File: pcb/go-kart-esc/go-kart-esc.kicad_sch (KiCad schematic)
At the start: 18 parts, among them J1 VBAT, J103 5V_CONN, J104 CAN_CONN, J105 SWD_CONN, J106 TEMP_CONN_A, J107 ENCODER_CONN_A, J108 ENCODER_CONN_B, J109 TEMP_CONN_B, J111 THROTTLE_CONN, J112 BRAKE_CONN, J3 GND

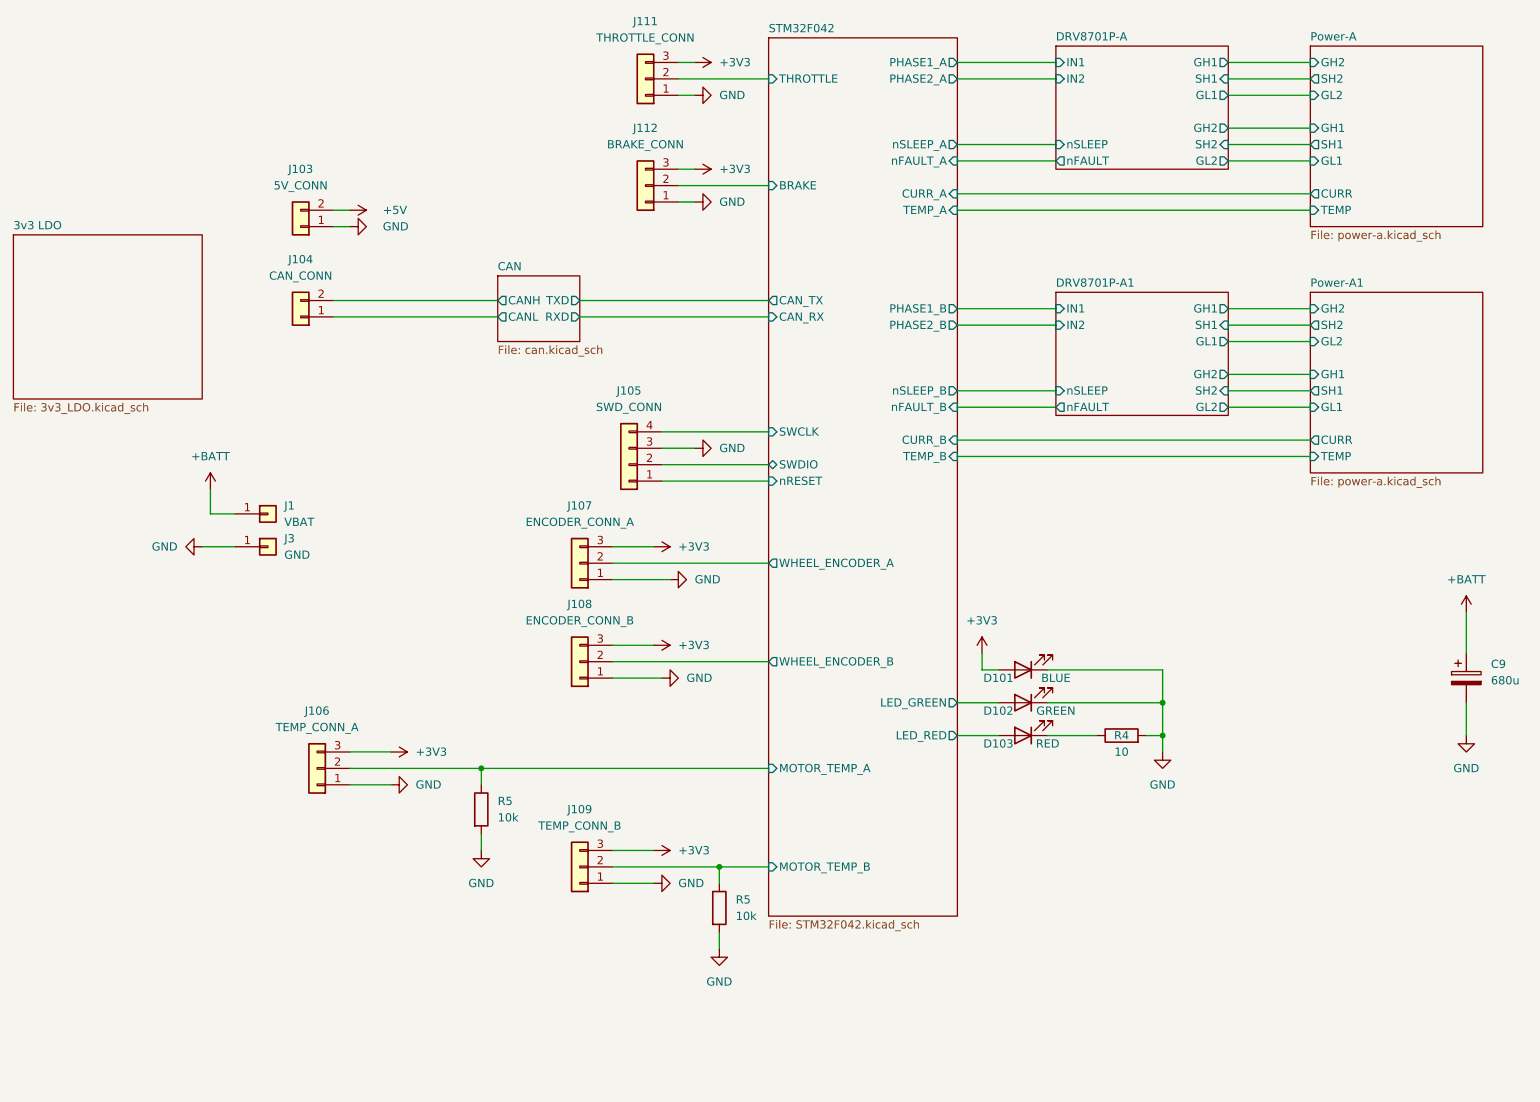
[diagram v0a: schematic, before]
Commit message: Theory can only take you so far.
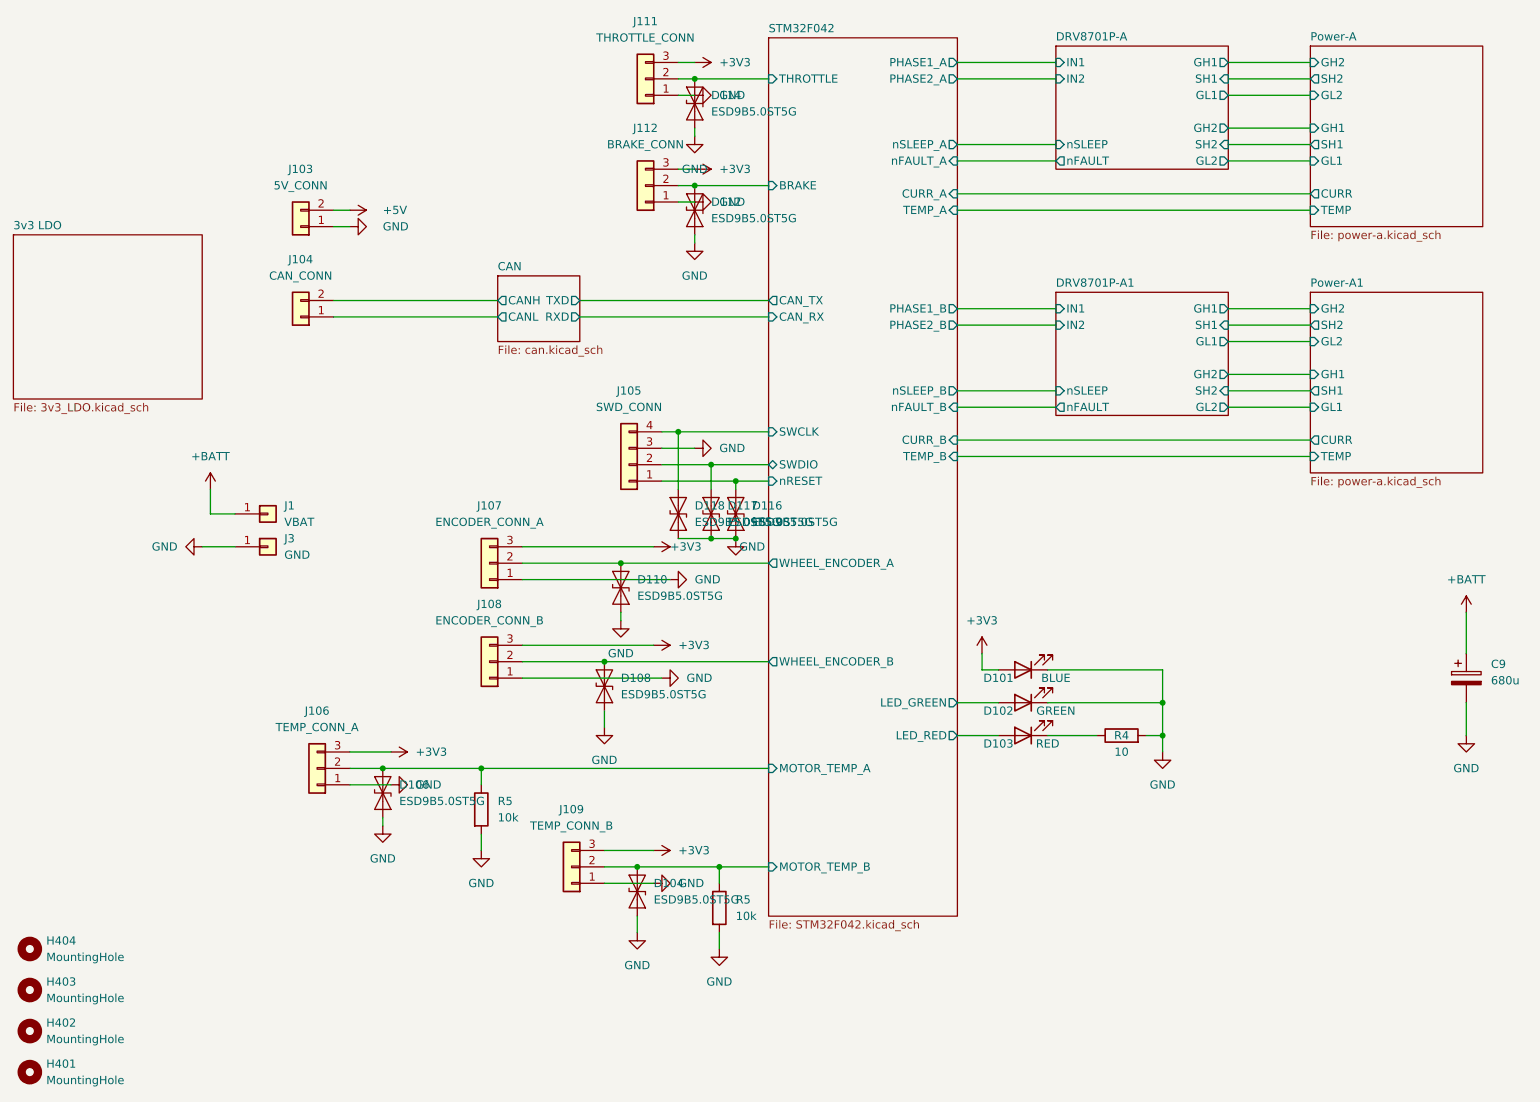
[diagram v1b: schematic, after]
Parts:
- added D104, D106, D108, D110, D112, D114, D116, D117, D118: ESD9B5.0ST5G, Diode_SMD:D_SOD-923, symbol Diode:ESD9B5.0ST5G
- added H401, H402, H403, H404: MountingHole, MountingHole:MountingHole_3.2mm_M3, symbol Mechanical:MountingHole
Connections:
- net GND: now also D104.1 (A1), D106.1 (A1), D108.1 (A1), D110.1 (A1), D112.1 (A1), D114.1 (A1), D116.1 (A1), D117.1 (A1), D118.1 (A1)
- net STM32F042/BRAKE: now also D112.2 (A2)
- net STM32F042/MOTOR_TEMP_A: now also D106.2 (A2)
- net STM32F042/MOTOR_TEMP_B: now also D104.2 (A2)
- net STM32F042/SWCLK: now also D118.2 (A2)
- net STM32F042/SWDIO: now also D117.2 (A2)
- net STM32F042/THROTTLE: now also D114.2 (A2)
- net STM32F042/WHEEL_ENCODER_A: now also D110.2 (A2)
- net STM32F042/WHEEL_ENCODER_B: now also D108.2 (A2)
- net STM32F042/nRESET: now also D116.2 (A2)
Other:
- moved on the sheet: J107, J108, J109
